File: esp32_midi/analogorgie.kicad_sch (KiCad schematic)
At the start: 62 parts, among them U10 BL1551, U11 BL1551, U12 BL1551, U13 BL1551, U14 BL1551, U15 BL1551, U16 BL1551, U17 BL1551, U18 BL1551, U19 BL1551, U20 BL1551, U21 BL1551, U22 BL1551, U23 BL1551, U24 BL1551, U25 BL1551, U26 BL1551, U27 BL1551, U28 BL1551, U29 BL1551, U30 BL1551, U31 BL1551, U32 BL1551, U33 BL1551, U34 BL1551, U35 BL1551, U6 BL1551, U7 BL1551, U8 BL1551, U9 BL1551

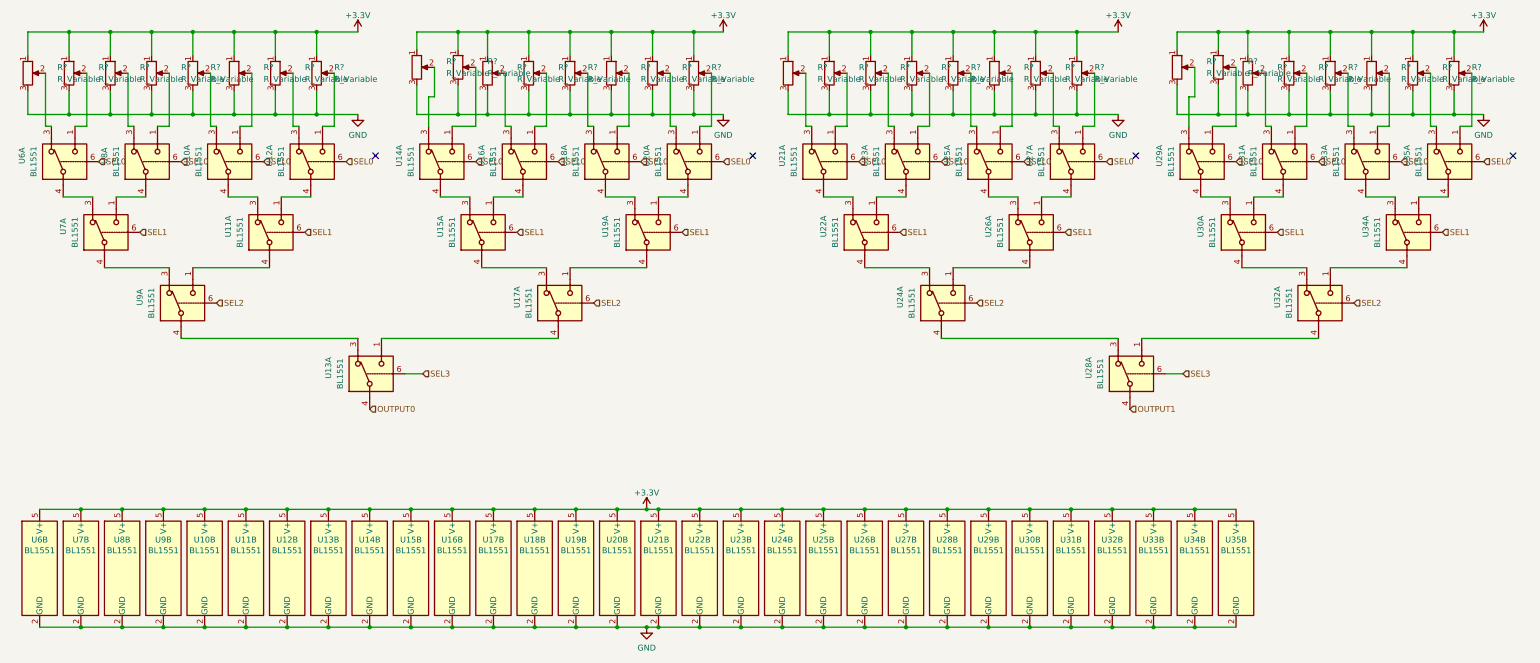
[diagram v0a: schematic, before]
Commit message: Add ordentliche-teile
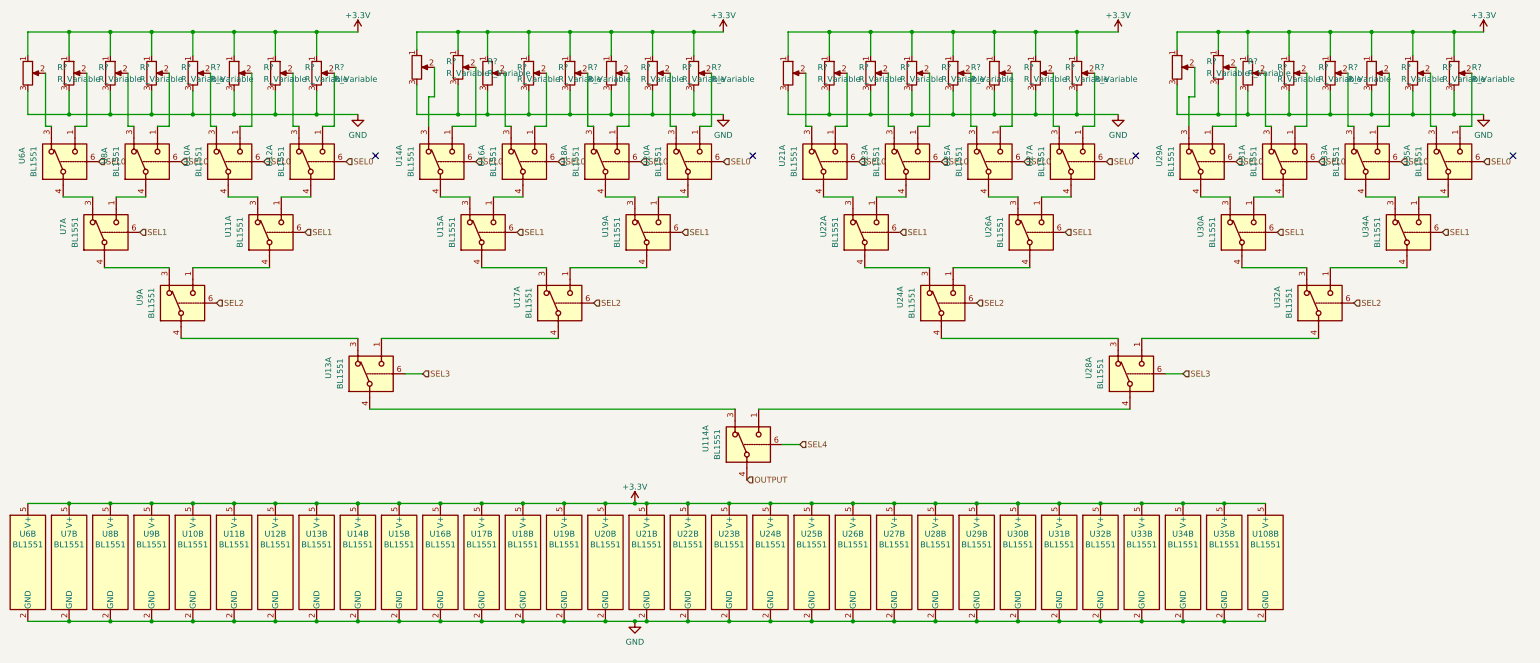
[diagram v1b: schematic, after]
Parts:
- added U108, U114: BL1551, Package_TO_SOT_SMD:SOT-363_SC-70-6, symbol Analog_Switch:FSA3157L6X
- R? (x8): footprint (none) -> ordentliche-teile:scheißfader
- R? (x24): footprint (none) -> Potentiometer_THT:Potentiometer_Alps_RK09L_Single_Vertical
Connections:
- net +3.3V: now also U108.5 (V+)
- net GND: now also U108.2 (GND)
- net OUTPUT0: no longer names the net of U13.4
- net OUTPUT0: now also U114.3
- net OUTPUT1: no longer names the net of U28.4
- net OUTPUT1: now also U114.1
- new net OUTPUT: U114.4
- new net SEL4: U114.6
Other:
- moved on the sheet: U10B, U11B, U12B, U13B, U14B, U15B, U16B, U17B, U18B, U19B, U20B, U21B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
